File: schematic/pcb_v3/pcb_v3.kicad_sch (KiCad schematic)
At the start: 59 parts, among them IC1 FT232RNQ-TRAY, J1 5V, J10 UART/SPI, J11 Conn_01x03_Pin, J2 SERVO, J3 MAVLINK, J4 DISPLAY, J5 SER. SERVO, J6 MAG., J7 U.FL-R, J8 Conn_01x05_Pin, J9 Conn_01x05_Pin, P1 USB_C_Plug_USB2.0, Q1 NPN, Q2 NPN, SW1 BOOT, SW2 SW_Push, SW3 SW_Push, SW4 SW_Push, SW5 SW_Push, SW6 RESET, U1 NEO-M9N, U2 AP7361C-33E, U3 FM24C64B

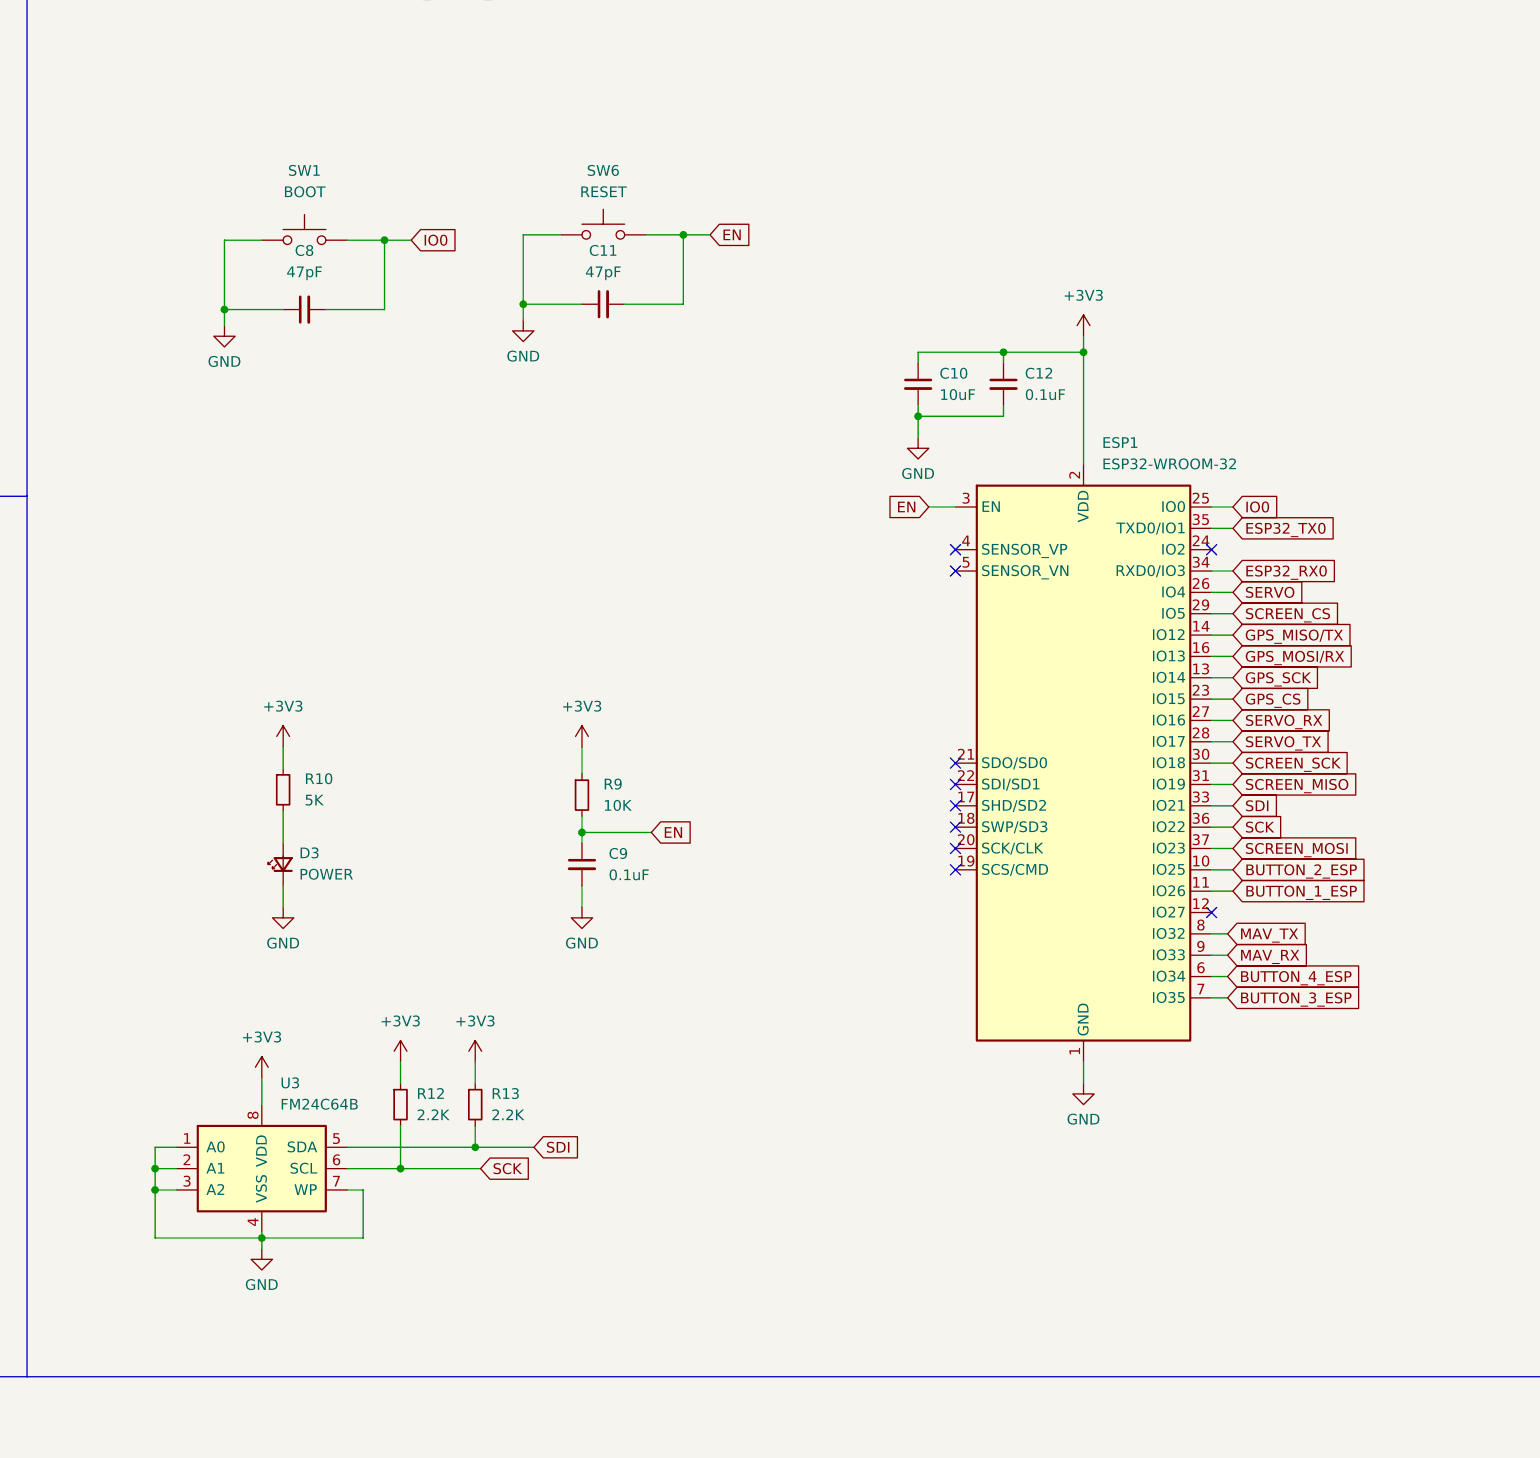
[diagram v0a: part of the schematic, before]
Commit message: pcb cleanup
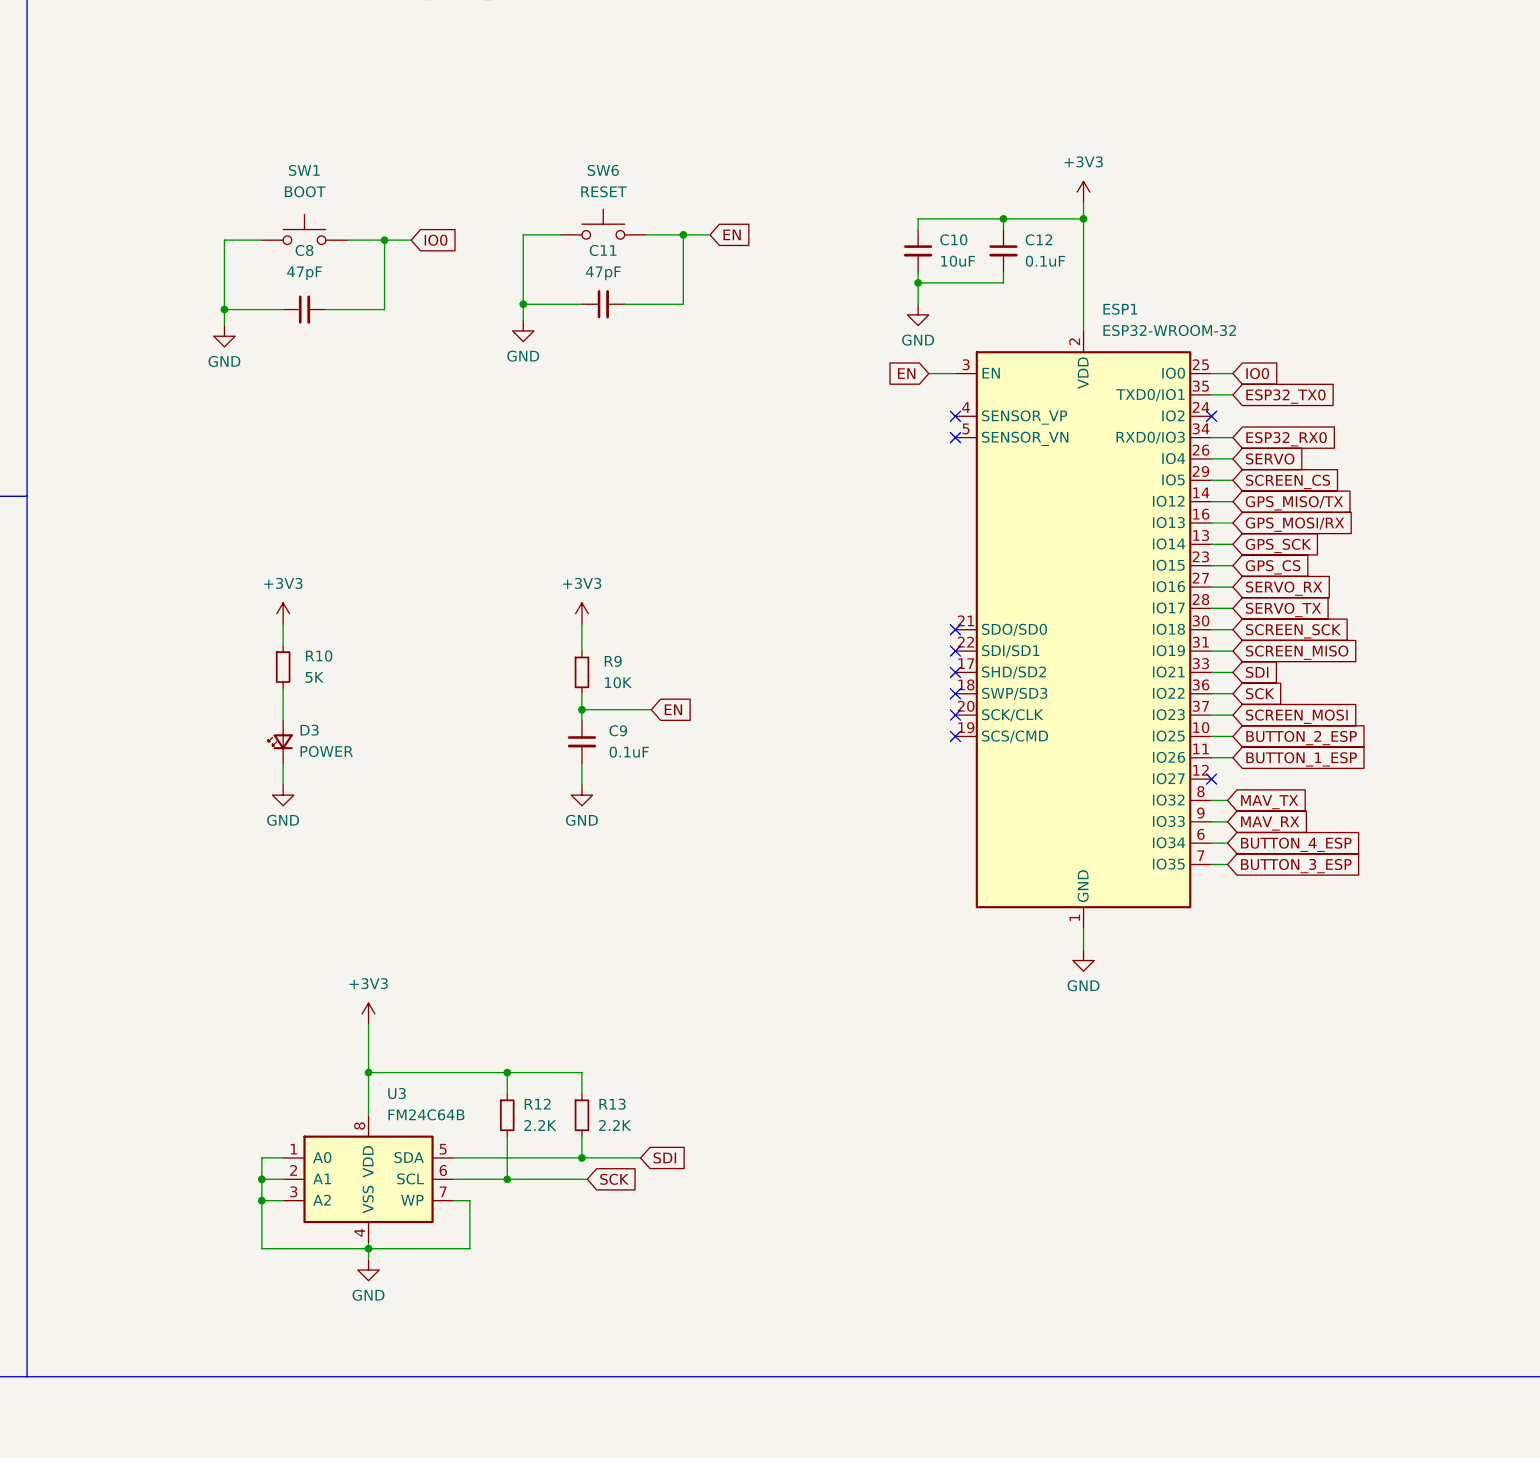
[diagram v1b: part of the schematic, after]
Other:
- moved on the sheet: C10, C12, C9, D3, ESP1, R10, R12, R13, R9, U3
